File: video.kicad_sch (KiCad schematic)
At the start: 40 parts, among them Q6 2N3904, U10 4164, U11 4164, U12 4164, U13 4164, U14 4164, U15 4164, U16 4164, U21 74LS74, U26 4164, U27 4164, U28 4164, U29 4164, U30 4164, U31 4164, U32 4164, U33 4164, U36 MMMU, U6 C061991/FREDDIE, U9 4164, Y2 4.33618MHz

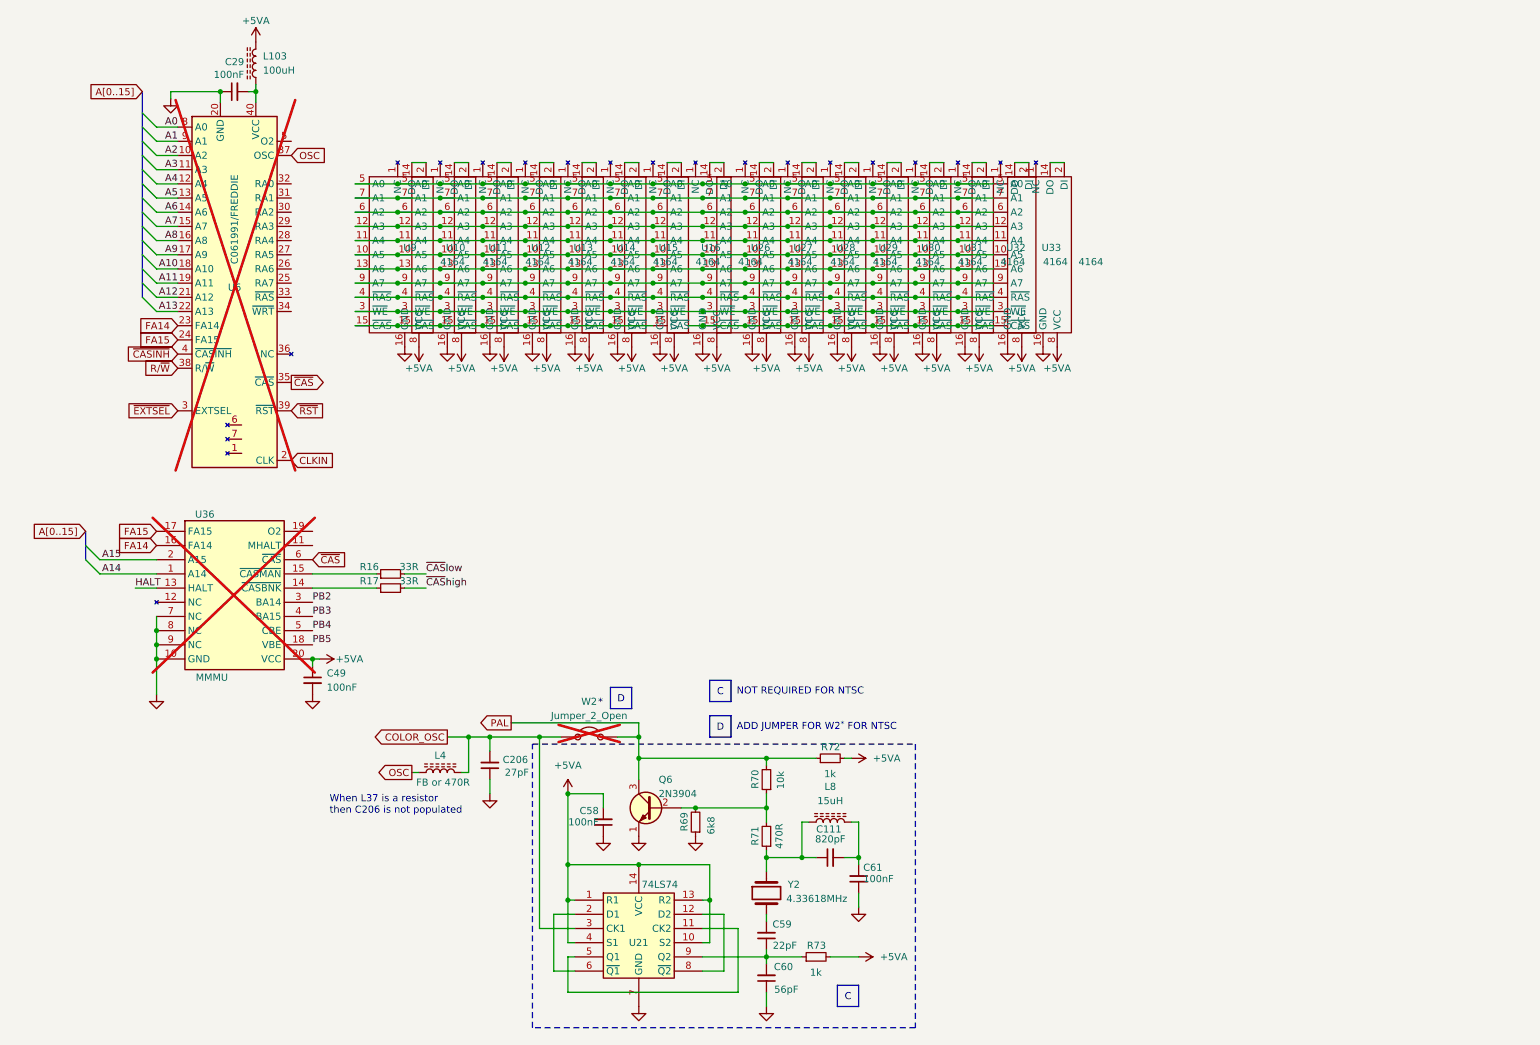
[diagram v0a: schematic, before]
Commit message: tidy up
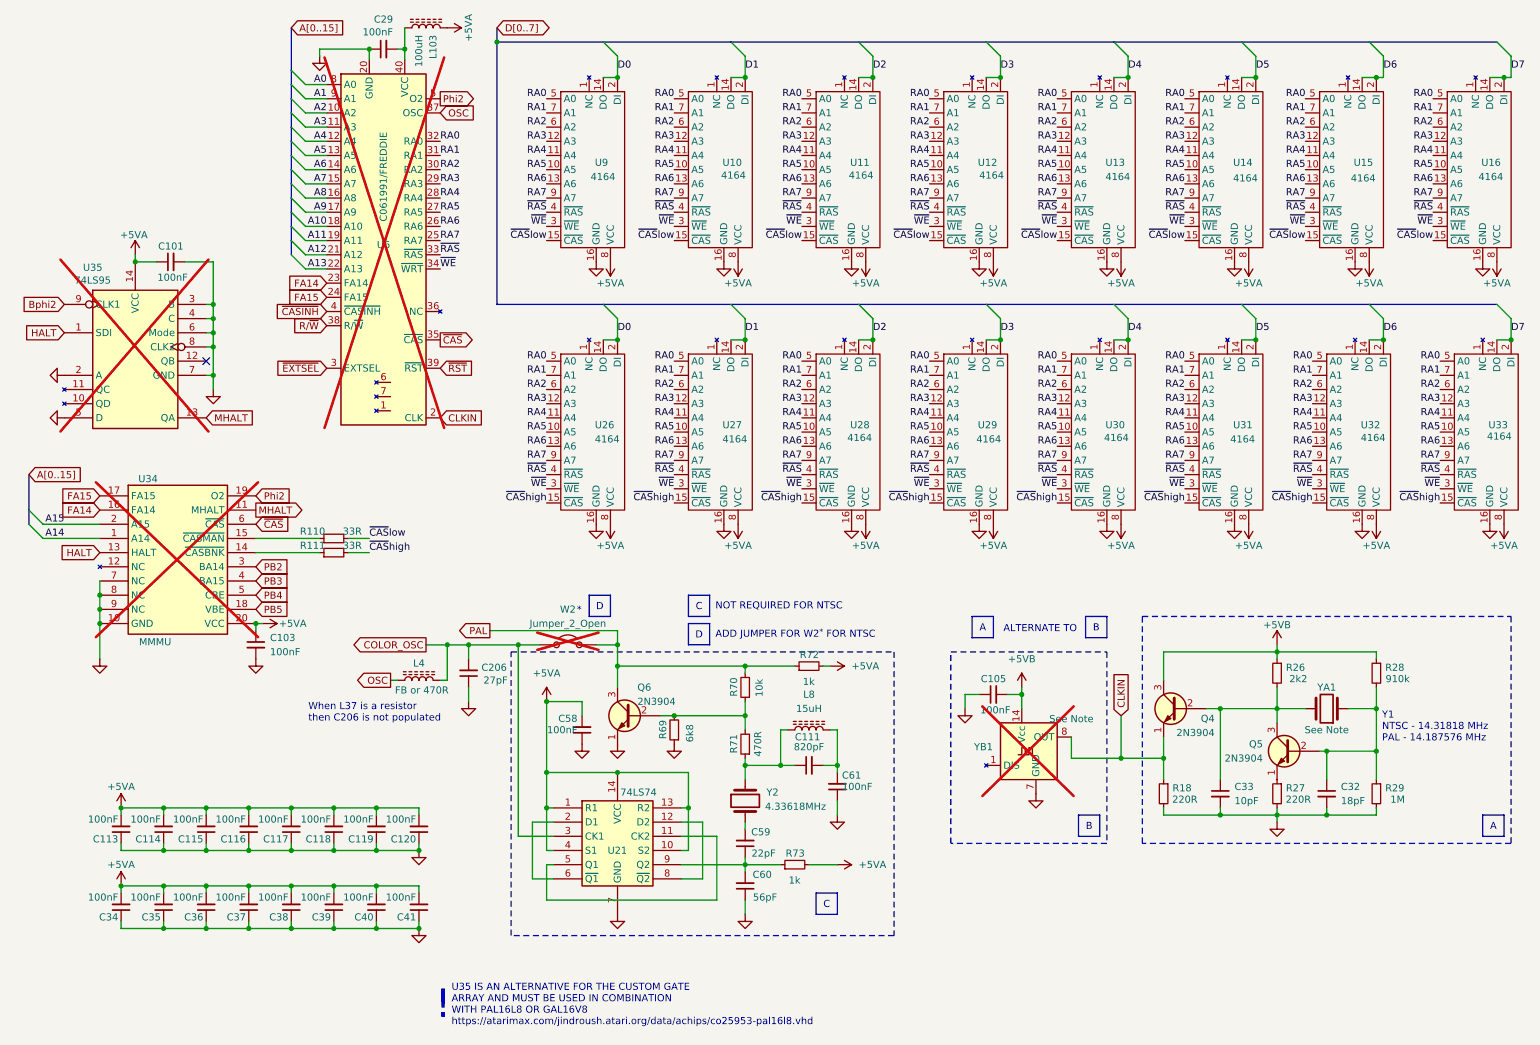
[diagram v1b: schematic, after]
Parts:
- added C101, C105: 100nF, Library:C_Axial_L5.1mm_D2.7mm_P12.72mm_Horizontal, symbol Device:C_Small
- added C113, C114, C115, C116, C117, C118, C119, C120, C34, C35, C36, C37, C38, C39, C40, C41: 100nF, Library:C_Axial_L3.8mm_D2.6mm_P8.89mm_Horizontal, symbol Device:C_Small
- added C32: 18pF, Library:C_Axial_L5.1mm_D2.7mm_P12.72mm_Horizontal, symbol Device:C_Small
- added C33: 10pF, Library:C_Axial_L5.1mm_D2.7mm_P12.72mm_Horizontal, symbol Device:C_Small
- added Q4, Q5: 2N3904, Library:TO-92L_Inline_Wide, symbol PCM_Transistor_BJT_AKL:2N3904
- added R18, R27: 220R, Library:R_Axial_L9.0mm_D2.7mm_P12.70mm_Horizontal, symbol Device:R_Small
- added R26: 2k2, Library:R_Axial_L9.0mm_D2.7mm_P12.70mm_Horizontal, symbol Device:R_Small
- added R28: 910k, Library:R_Axial_L9.0mm_D2.7mm_P12.70mm_Horizontal, symbol Device:R_Small
- added R29: 1M, Library:R_Axial_L9.0mm_D2.7mm_P12.70mm_Horizontal, symbol Device:R_Small
- added U35: 74LS95, Package_DIP:DIP-14_W7.62mm, symbol Library:74LS95
- added YA1: See Note, Crystal:Crystal_HC49-U_Horizontal, symbol PCM_Crystal_AKL:Crystal_Generic
- added YB1: See Note, Oscillator:Oscillator_DIP-14, symbol Library:CXO-DIP14
- renumbered C49 to C103, R16 to R110, R17 to R111, U36 to U34
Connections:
- net +5VA: now also C101.1, C113.2, C114.2, C115.2, C116.2, C117.2, C118.2, C119.2, C120.2, C34.2, C35.2, C36.2, C37.2, C38.2, C39.2, C40.2, C41.2, U35.14 (VCC)
- net CLKIN: now also Q4.1 (E), R18.1, YB1.8 (OUT)
- net GND: now also C101.2, C105.1, C113.1, C114.1, C115.1, C116.1, C117.1, C118.1, C119.1, C120.1, C32.2, C33.2, C34.1, C35.1, C36.1, C37.1, C38.1, C39.1, C40.1, C41.1, R18.2, R27.2, R29.2, U35.2 (A), U35.3 (B), U35.4 (C), U35.5 (D), U35.6 (Mode), U35.7 (GND), U35.8 (CLK2), YB1.7 (GND)
- net HALT: now also U35.1 (SDI)
- net ~{CAS}high: now also U26.15 (~{CAS}), U27.15 (~{CAS}), U28.15 (~{CAS}), U29.15 (~{CAS}), U30.15 (~{CAS}), U31.15 (~{CAS}), U32.15 (~{CAS}), U33.15 (~{CAS})
- net ~{CAS}low: now also U10.15 (~{CAS}), U11.15 (~{CAS}), U12.15 (~{CAS}), U13.15 (~{CAS}), U14.15 (~{CAS}), U15.15 (~{CAS}), U16.15 (~{CAS}), U9.15 (~{CAS})
- net RA5: now reaches U10.10 (A5), U11.10 (A5), U12.10 (A5), U13.10 (A5), U14.10 (A5), U15.10 (A5), U16.10 (A5), U26.10 (A5), U27.10 (A5), U28.10 (A5), U29.10 (A5), U30.10 (A5), U31.10 (A5), U32.10 (A5), U33.10 (A5), U9.10 (A5)
- net RA5: now also U6.27 (RA5)
- net RA4: now reaches U10.11 (A4), U11.11 (A4), U12.11 (A4), U13.11 (A4), U14.11 (A4), U15.11 (A4), U16.11 (A4), U26.11 (A4), U27.11 (A4), U28.11 (A4), U29.11 (A4), U30.11 (A4), U31.11 (A4), U32.11 (A4), U33.11 (A4), U9.11 (A4)
- net RA4: now also U6.28 (RA4)
- net RA3: now reaches U10.12 (A3), U11.12 (A3), U12.12 (A3), U13.12 (A3), U14.12 (A3), U15.12 (A3), U16.12 (A3), U26.12 (A3), U27.12 (A3), U28.12 (A3), U29.12 (A3), U30.12 (A3), U31.12 (A3), U32.12 (A3), U33.12 (A3), U9.12 (A3)
- net RA3: now also U6.29 (RA3)
- net RA6: now reaches U10.13 (A6), U11.13 (A6), U12.13 (A6), U13.13 (A6), U14.13 (A6), U15.13 (A6), U16.13 (A6), U26.13 (A6), U27.13 (A6), U28.13 (A6), U29.13 (A6), U30.13 (A6), U31.13 (A6), U32.13 (A6), U33.13 (A6), U9.13 (A6)
- net RA6: now also U6.26 (RA6)
- net D2: now reaches U28.14 (DO), U28.2 (DI)
- net D2: now also U11.14 (DO), U11.2 (DI)
- net ~{WE}: now reaches U10.3 (~{WE}), U11.3 (~{WE}), U12.3 (~{WE}), U13.3 (~{WE}), U14.3 (~{WE}), U15.3 (~{WE}), U16.3 (~{WE}), U26.3 (~{WE}), U27.3 (~{WE}), U28.3 (~{WE}), U29.3 (~{WE}), U30.3 (~{WE}), U31.3 (~{WE}), U32.3 (~{WE}), U33.3 (~{WE}), U9.3 (~{WE})
- net ~{WE}: now also U6.34 (~{WRT})
- net ~{RAS}: now reaches U10.4 (~{RAS}), U11.4 (~{RAS}), U12.4 (~{RAS}), U13.4 (~{RAS}), U14.4 (~{RAS}), U15.4 (~{RAS}), U16.4 (~{RAS}), U26.4 (~{RAS}), U27.4 (~{RAS}), U28.4 (~{RAS}), U29.4 (~{RAS}), U30.4 (~{RAS}), U31.4 (~{RAS}), U32.4 (~{RAS}), U33.4 (~{RAS}), U9.4 (~{RAS})
- net ~{RAS}: now also U6.33 (~{RAS})
- net RA0: now reaches U10.5 (A0), U11.5 (A0), U12.5 (A0), U13.5 (A0), U14.5 (A0), U15.5 (A0), U16.5 (A0), U26.5 (A0), U27.5 (A0), U28.5 (A0), U29.5 (A0), U30.5 (A0), U31.5 (A0), U32.5 (A0), U33.5 (A0), U9.5 (A0)
- net RA0: now also U6.32 (RA0)
- net RA2: now reaches U10.6 (A2), U11.6 (A2), U12.6 (A2), U13.6 (A2), U14.6 (A2), U15.6 (A2), U16.6 (A2), U26.6 (A2), U27.6 (A2), U28.6 (A2), U29.6 (A2), U30.6 (A2), U31.6 (A2), U32.6 (A2), U33.6 (A2), U9.6 (A2)
- net RA2: now also U6.30 (RA2)
- net RA1: now reaches U10.7 (A1), U11.7 (A1), U12.7 (A1), U13.7 (A1), U14.7 (A1), U15.7 (A1), U16.7 (A1), U26.7 (A1), U27.7 (A1), U28.7 (A1), U29.7 (A1), U30.7 (A1), U31.7 (A1), U32.7 (A1), U33.7 (A1), U9.7 (A1)
- net RA1: now also U6.31 (RA1)
- net RA7: now reaches U10.9 (A7), U11.9 (A7), U12.9 (A7), U13.9 (A7), U14.9 (A7), U15.9 (A7), U16.9 (A7), U26.9 (A7), U27.9 (A7), U28.9 (A7), U29.9 (A7), U30.9 (A7), U31.9 (A7), U32.9 (A7), U33.9 (A7), U9.9 (A7)
- net RA7: now also U6.25 (RA7)
- net D1: now reaches U10.14 (DO), U10.2 (DI)
- net D1: now also U27.14 (DO), U27.2 (DI)
- net D5: now reaches U14.14 (DO), U14.2 (DI)
- net D5: now also U31.14 (DO), U31.2 (DI)
- net D0: now reaches U26.14 (DO), U26.2 (DI)
- net D0: now also U9.14 (DO), U9.2 (DI)
- net D4: now reaches U13.14 (DO), U13.2 (DI)
- net D4: now also U30.14 (DO), U30.2 (DI)
- net Phi2: now reaches U6.5 (O2)
- net Phi2: now also U34.19 (O2)
- net D6: now reaches U15.14 (DO), U15.2 (DI)
- net D6: now also U32.14 (DO), U32.2 (DI)
- net D7: now reaches U16.14 (DO), U16.2 (DI)
- net D7: now also U33.14 (DO), U33.2 (DI)
- net D3: now reaches U29.14 (DO), U29.2 (DI)
- net D3: now also U12.14 (DO), U12.2 (DI)
- net MHALT: now reaches U34.11 (MHALT)
- net MHALT: now also U35.13 (QA)
- new net: C32.1, Q5.2 (B), R28.2, R29.1, YA1.1
- new net: C33.1, Q4.2 (B), Q5.3 (C), R26.2, YA1.2
- new net: Q5.1 (E), R27.1
- new net +5VB: C105.2, Q4.3 (C), R26.1, R28.1, YB1.14 (Vcc)
- new net Bphi2: U35.9 (CLK1)
- no-connect marks 0 -> 1
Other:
- note added: "!"
- note added: "ALTERNATE TO"
- note added: "U35 IS AN ALTERNATIVE FOR THE CUSTOM GATE ARRAY AND MUST BE USED IN COMBINATION WITH PAL16L8 OR GAL16V8 https://atarimax.com/jindroush.atari.org/data/achips/co25953-pal16l8.vhd"
- note added: "Y1 NTSC - 14.31818 MHz PAL - 14.187576 MHz"
- moved on the sheet: C103, C111, C206, C29, C58, C59, C60, C61, L103, L4, L8, Q6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
